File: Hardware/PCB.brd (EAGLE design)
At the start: 46 x 34.8 mm, 105 parts, among them IC1 BQ25180YBGR_BQ25180YBGR, IC2 DRV2605YZFR, IC3 BMA421, IC9 RT6160AWSC, J1 503480-2400, J2 TC2030-IDC, J4 KH-TYPE-C-16P, Q1 20V/4.2A/52mΩ/1.4W, Q3 SI1308EDL-T1-GE3, U1 NRF52840_QF, U3 MAX17048G+T10, X1 32MHz, X2 32.768kHz

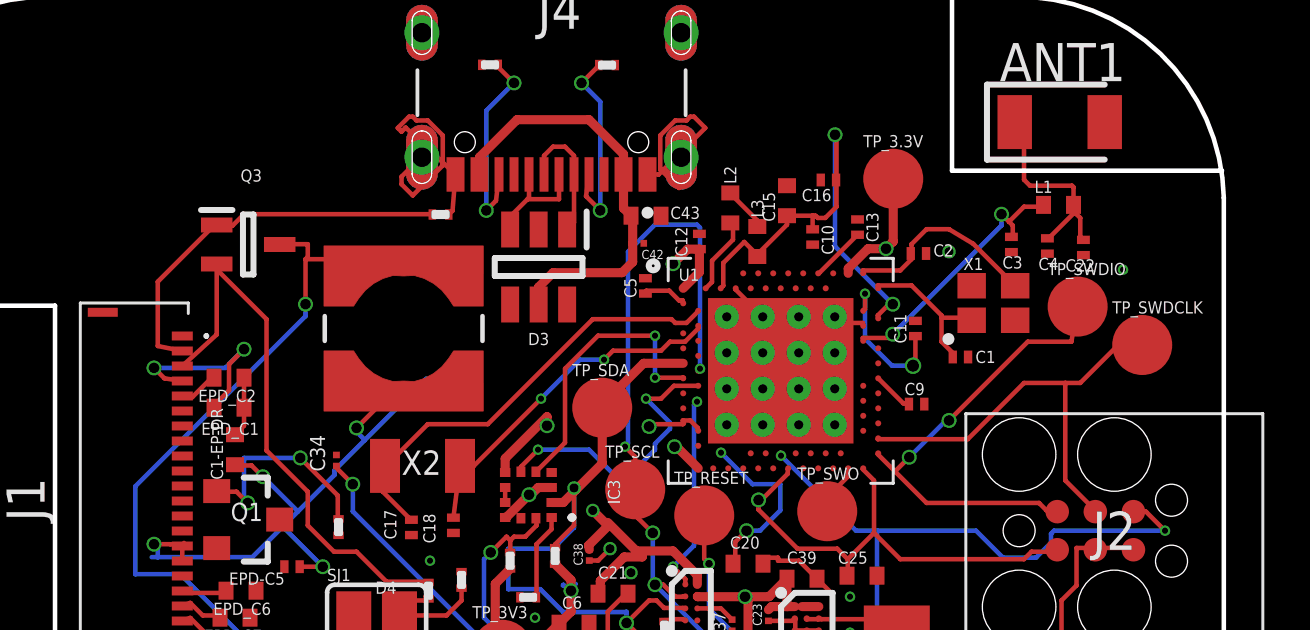
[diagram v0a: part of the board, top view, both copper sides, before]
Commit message: PCB v3
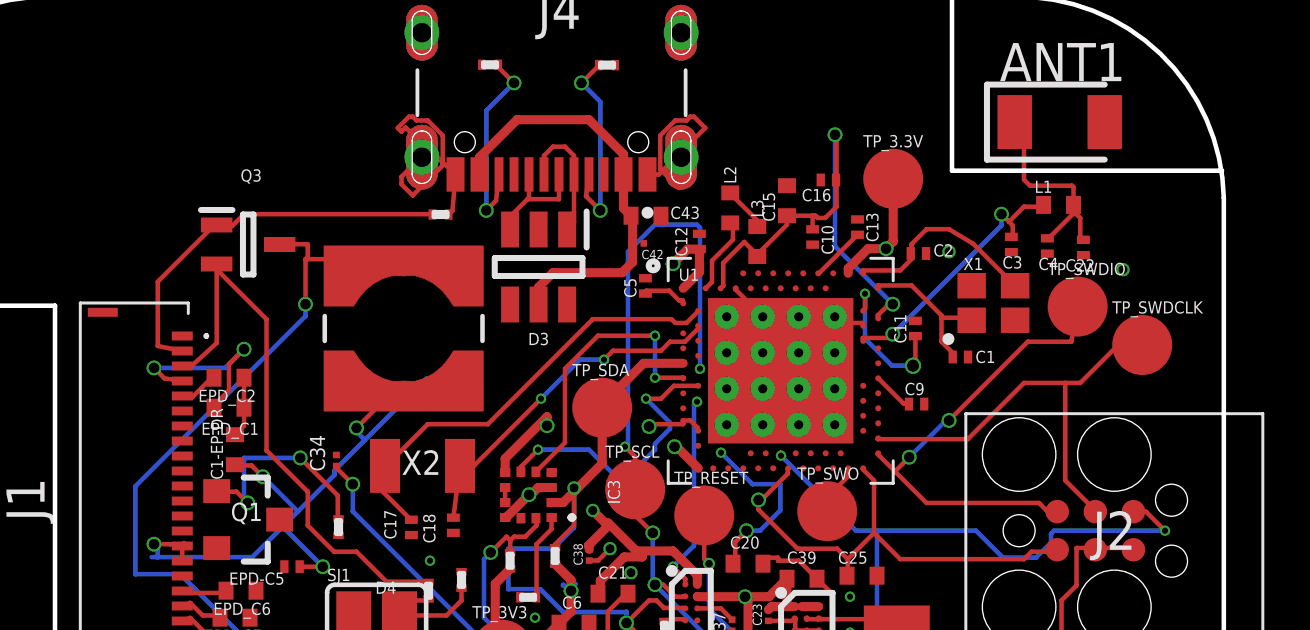
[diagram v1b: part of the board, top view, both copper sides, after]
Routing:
- net 3V3/2.4A: track 98.0 -> 99.8 mm
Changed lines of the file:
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@@
 <layer number="14" name="Route14" color="22" fill="1" visible="no" active="no"/>
 <layer number="15" name="Route15" color="23" fill="1" visible="yes" active="yes"/>
-<layer number="16" name="Bottom" color="1" fill="1" visible="no" active="yes"/>
+<layer number="16" name="Bottom" color="1" fill="1" visible="yes" active="yes"/>
 <layer number="17" name="Pads" color="2" fill="1" visible="no" active="yes"/>
 <layer number="18" name="Vias" color="2" fill="1" visible="yes" active="yes"/>
@@
 <via x="164.5" y="-230" extent="1-16" drill="0.3" alwaysstop="yes">
 </via>
-<via x="170.3" y="-230.6" extent="1-16" drill="0.2" alwaysstop="yes">
+<via x="170.3" y="-230.6" extent="1-16" drill="0.3" alwaysstop="yes">
 </via>
 <wire x1="149.705" y1="-237.86" x2="149.705" y2="-238.36" width="0.1524" layer="1"/>
@@
 <via x="151.1" y="-235.8" extent="1-16" drill="0.35" alwaysstop="yes">
 </via>
-<wire x1="150.5" y1="-238.1" x2="150.5" y2="-236.4" width="0.3048" layer="15"/>
-<wire x1="150.5" y1="-236.4" x2="151.1" y2="-235.8" width="0.3048" layer="15"/>
+<wire x1="150.2" y1="-236.2" x2="150.2" y2="-237.8" width="0.3048" layer="15"/>
+<wire x1="150.5" y1="-238.1" x2="150.2" y2="-237.8" width="0.3048" layer="15"/>
+<wire x1="150.6" y1="-235.8" x2="151.1" y2="-235.8" width="0.3048" layer="15"/>
+<wire x1="150.6" y1="-235.8" x2="150.2" y2="-236.2" width="0.3048" layer="15"/>
 <wire x1="149.87" y1="-240.575" x2="149.375" y2="-241.07" width="0.3048" layer="1"/>
 <wire x1="149.375" y1="-241.07" x2="149.375" y2="-243.125" width="0.3048" layer="1"/>
@@
 <wire x1="157.8" y1="-247.1" x2="159.375" y2="-245.525" width="0.3048" layer="15"/>
 <wire x1="159.375" y1="-245.525" x2="159.375" y2="-244.125" width="0.3048" layer="15"/>
-<wire x1="159.375" y1="-244.125" x2="159.375" y2="-239.5" width="0.3048" layer="15"/>
-<wire x1="159.375" y1="-239.5" x2="158.15" y2="-238.275" width="0.3048" layer="15"/>
+<wire x1="159.975" y1="-240.1" x2="159.975" y2="-243.525" width="0.3048" layer="15"/>
+<wire x1="159.375" y1="-244.125" x2="159.975" y2="-243.525" width="0.3048" layer="15"/>
+<wire x1="159.975" y1="-240.1" x2="158.15" y2="-238.275" width="0.3048" layer="15"/>
 <wire x1="155.3" y1="-230.4" x2="155.3" y2="-235.025" width="0.3048" layer="15"/>
 <wire x1="155.3" y1="-235.025" x2="155.3" y2="-235.425" width="0.3048" layer="15"/>
-<wire x1="155.3" y1="-235.425" x2="158.15" y2="-238.275" width="0.3048" layer="15"/>
 <wire x1="154.5" y1="-235.825" x2="155.3" y2="-235.025" width="0.3048" layer="15"/>
 <wire x1="151.1" y1="-235.8" x2="151.1" y2="-235.500009375" width="0.3048" layer="1"/>
@@
 <wire x1="151.5" y1="-242.4" x2="151.9" y2="-242" width="0.3048" layer="1"/>
 <wire x1="151.9" y1="-242" x2="151.9" y2="-241.3" width="0.3048" layer="1"/>
+<wire x1="158.15" y1="-238.275" x2="157.175" y2="-237.3" width="0.3048" layer="15"/>
+<wire x1="157.175" y1="-237.3" x2="156.5" y2="-237.3" width="0.3048" layer="15"/>
+<wire x1="156.5" y1="-237.3" x2="156.4" y2="-237.4" width="0.3048" layer="15"/>
+<wire x1="156.4" y1="-237.4" x2="156" y2="-237" width="0.3048" layer="15"/>
+<wire x1="156" y1="-237" x2="156" y2="-236.9" width="0.3048" layer="15"/>
+<wire x1="156" y1="-236.9" x2="156.2" y2="-236.7" width="0.3048" layer="15"/>
+<wire x1="156.2" y1="-236.7" x2="156.2" y2="-236.325" width="0.3048" layer="15"/>
+<wire x1="156.2" y1="-236.325" x2="155.3" y2="-235.425" width="0.3048" layer="15"/>
 </signal>
 <signal name="N$2">
@@
 <wire x1="147.125" y1="-241" x2="147.15" y2="-241.025" width="0.1524" layer="1"/>
 <wire x1="140" y1="-230.5" x2="140.09" y2="-230.41" width="0.1524" layer="1"/>
-<wire x1="140.09" y1="-230.41" x2="140.09" y2="-232.7622" width="0.1524" layer="1"/>
-<wire x1="140.09" y1="-232.7622" x2="138.9422" y2="-233.81" width="0.1524" layer="1"/>
+<wire x1="140.09" y1="-230.41" x2="140.09" y2="-233.044775" width="0.1524" layer="1"/>
+<wire x1="140.09" y1="-233.044775" x2="139.25174375" y2="-233.81" width="0.1524" layer="1"/>
+<wire x1="139.25174375" y1="-233.81" x2="138.9422" y2="-233.81" width="0.1524" layer="1"/>
 </signal>
 <signal name="N$29">
